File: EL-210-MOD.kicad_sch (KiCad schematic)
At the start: 2 parts, among them P1 EL-210-KEY, U1 9-ST-20

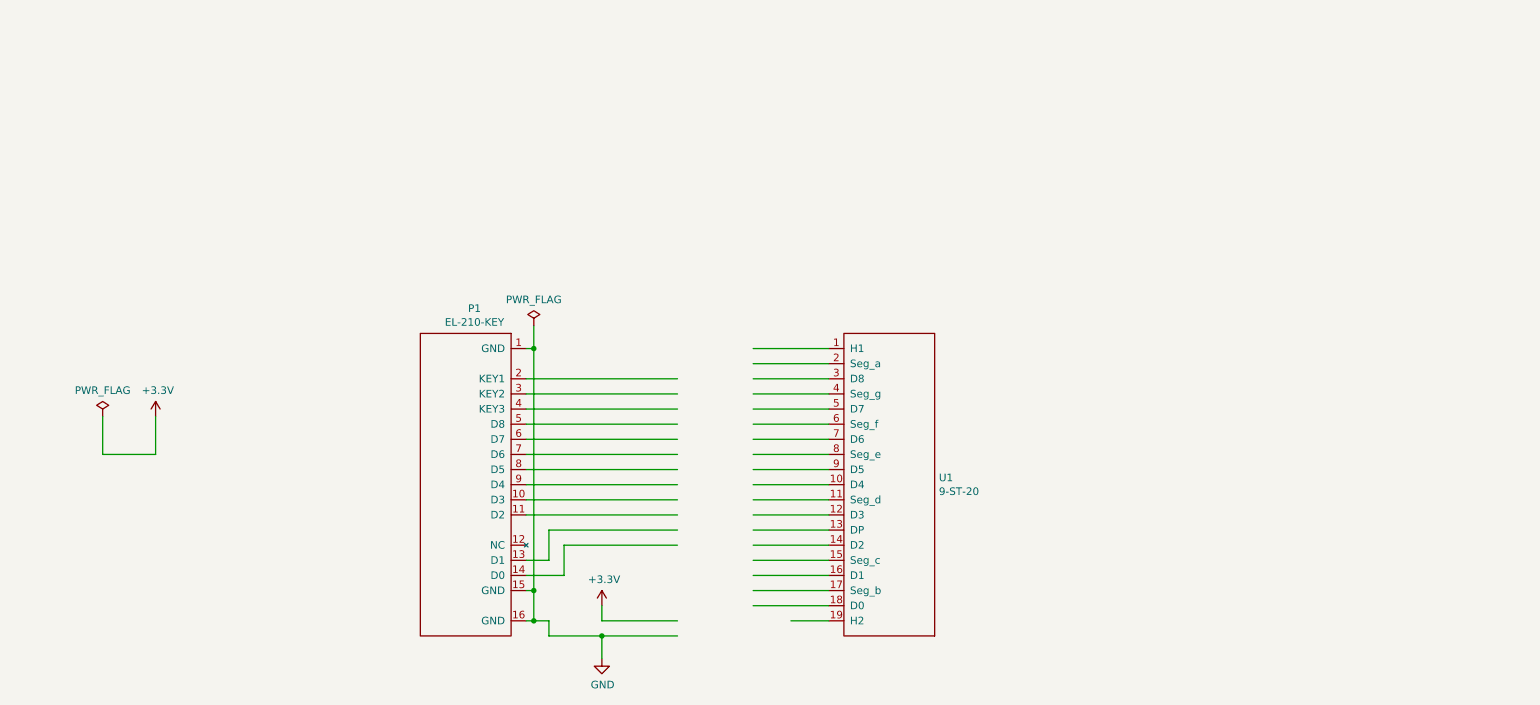
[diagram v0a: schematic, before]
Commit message: Rough layout of the digital part.
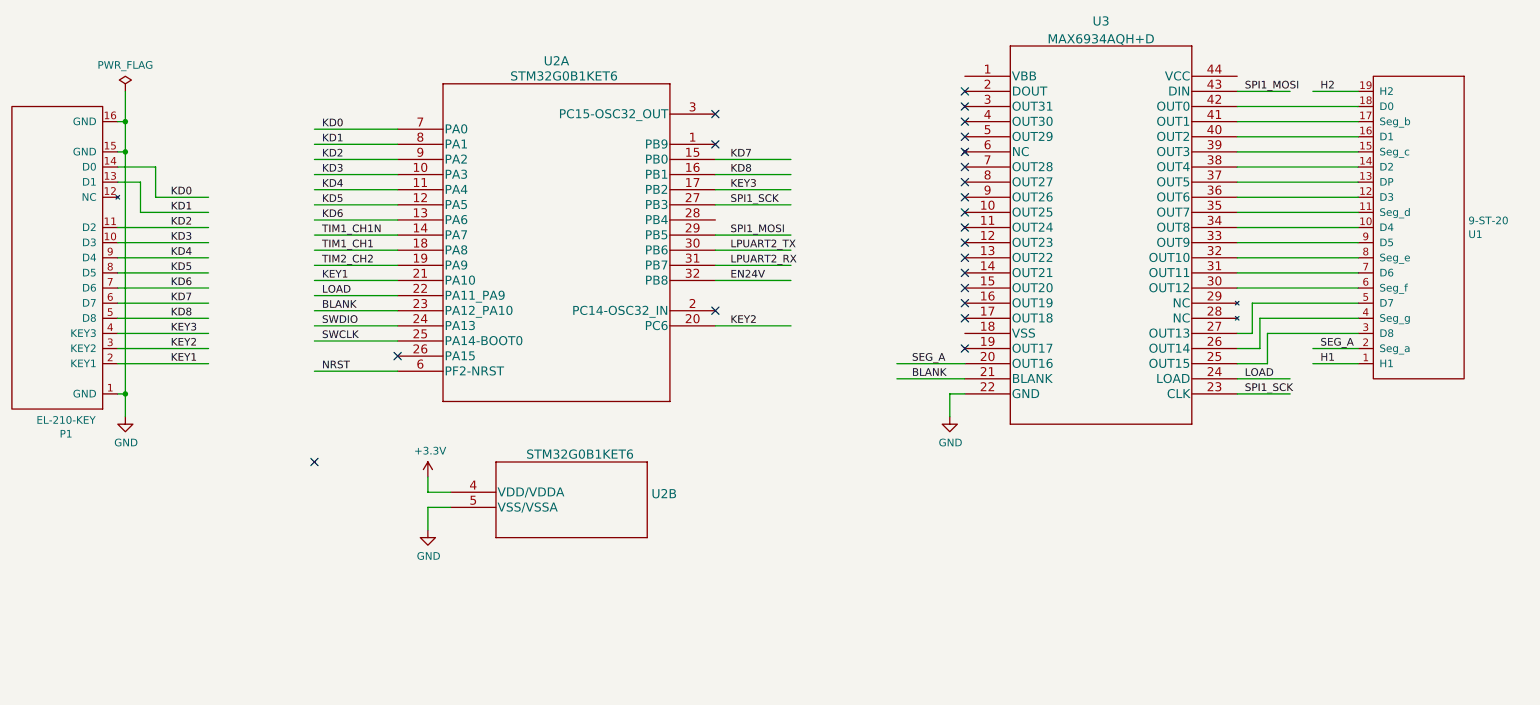
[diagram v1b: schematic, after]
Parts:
- added U2: STM32G0B1KET6, Package_QFP:LQFP-32_7x7mm_P0.8mm, symbol STM32G0B1KET6:STM32G0B1KET6
- added U3: MAX6934AQH+D, Package_LCC:PLCC-44, symbol MAX6934A:MAX6934AQH+D
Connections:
- net +3V3: now also U2.4 (VDD/VDDA)
- net GND: now also U2.5 (VSS/VSSA), U3.22 (GND)
- net KD3: now reaches P1.10 (D3)
- net KD3: now also U2.10 (PA3)
- net KD2: now reaches P1.11 (D2)
- net KD2: now also U2.9 (PA2)
- net KD1: now reaches P1.13 (D1)
- net KD1: now also U2.8 (PA1)
- net KD0: now reaches P1.14 (D0)
- net KD0: now also U2.7 (PA0)
- net KEY1: now reaches P1.2 (KEY1)
- net KEY1: now also U2.21 (PA10)
- net KEY2: now reaches P1.3 (KEY2)
- net KEY2: now also U2.20 (PC6)
- net KEY3: now reaches P1.4 (KEY3)
- net KEY3: now also U2.17 (PB2)
- net KD8: now reaches P1.5 (D8)
- net KD8: now also U2.16 (PB1)
- net KD7: now reaches P1.6 (D7)
- net KD7: now also U2.15 (PB0)
- net KD6: now reaches P1.7 (D6)
- net KD6: now also U2.13 (PA6)
- net KD5: now reaches P1.8 (D5)
- net KD5: now also U2.12 (PA5)
- net KD4: now reaches P1.9 (D4)
- net KD4: now also U2.11 (PA4)
- net H1: now reaches U1.1 (H1)
- net at U1.10 (D4): now also U3.34 (OUT8)
- net at U1.11 (Seg_d): now also U3.35 (OUT7)
- net at U1.12 (D3): now also U3.36 (OUT6)
- net at U1.13 (DP): now also U3.37 (OUT5)
- net at U1.14 (D2): now also U3.38 (OUT4)
- net at U1.15 (Seg_c): now also U3.39 (OUT3)
- net at U1.16 (D1): now also U3.40 (OUT2)
- net at U1.17 (Seg_b): now also U3.41 (OUT1)
- net at U1.18 (D0): now also U3.42 (OUT0)
- net H2: now reaches U1.19 (H2)
- net SEG_A: now reaches U1.2 (Seg_a)
- net SEG_A: now also U3.20 (OUT16)
- net at U1.3 (D8): now also U3.25 (OUT15)
- net at U1.4 (Seg_g): now also U3.26 (OUT14)
- net at U1.5 (D7): now also U3.27 (OUT13)
- net at U1.6 (Seg_f): now also U3.30 (OUT12)
- net at U1.7 (D6): now also U3.31 (OUT11)
- net at U1.8 (Seg_e): now also U3.32 (OUT10)
- net at U1.9 (D5): now also U3.33 (OUT9)
- new net BLANK: U2.23 (PA12_PA10), U3.21 (BLANK)
- new net EN24V: U2.32 (PB8)
- new net LOAD: U2.22 (PA11_PA9), U3.24 (LOAD)
- new net LPUART2_RX: U2.31 (PB7)
- new net LPUART2_TX: U2.30 (PB6)
- new net NRST: U2.6 (PF2-NRST)
- new net SPI1_MOSI: U2.29 (PB5), U3.43 (DIN)
- new net SPI1_SCK: U2.27 (PB3), U3.23 (CLK)
- new net SWCLK: U2.25 (PA14-BOOT0)
- new net SWDIO: U2.24 (PA13)
- new net TIM1_CH1: U2.18 (PA8)
- new net TIM1_CH1N: U2.14 (PA7)
- new net TIM2_CH2: U2.19 (PA9)
- no-connect marks 0 -> 22
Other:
- moved on the sheet: P1, U1
